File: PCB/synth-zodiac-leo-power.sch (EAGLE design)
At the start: 29 parts, among them J1 2.5 ID x 5.5 OD, J2 HDR-02P

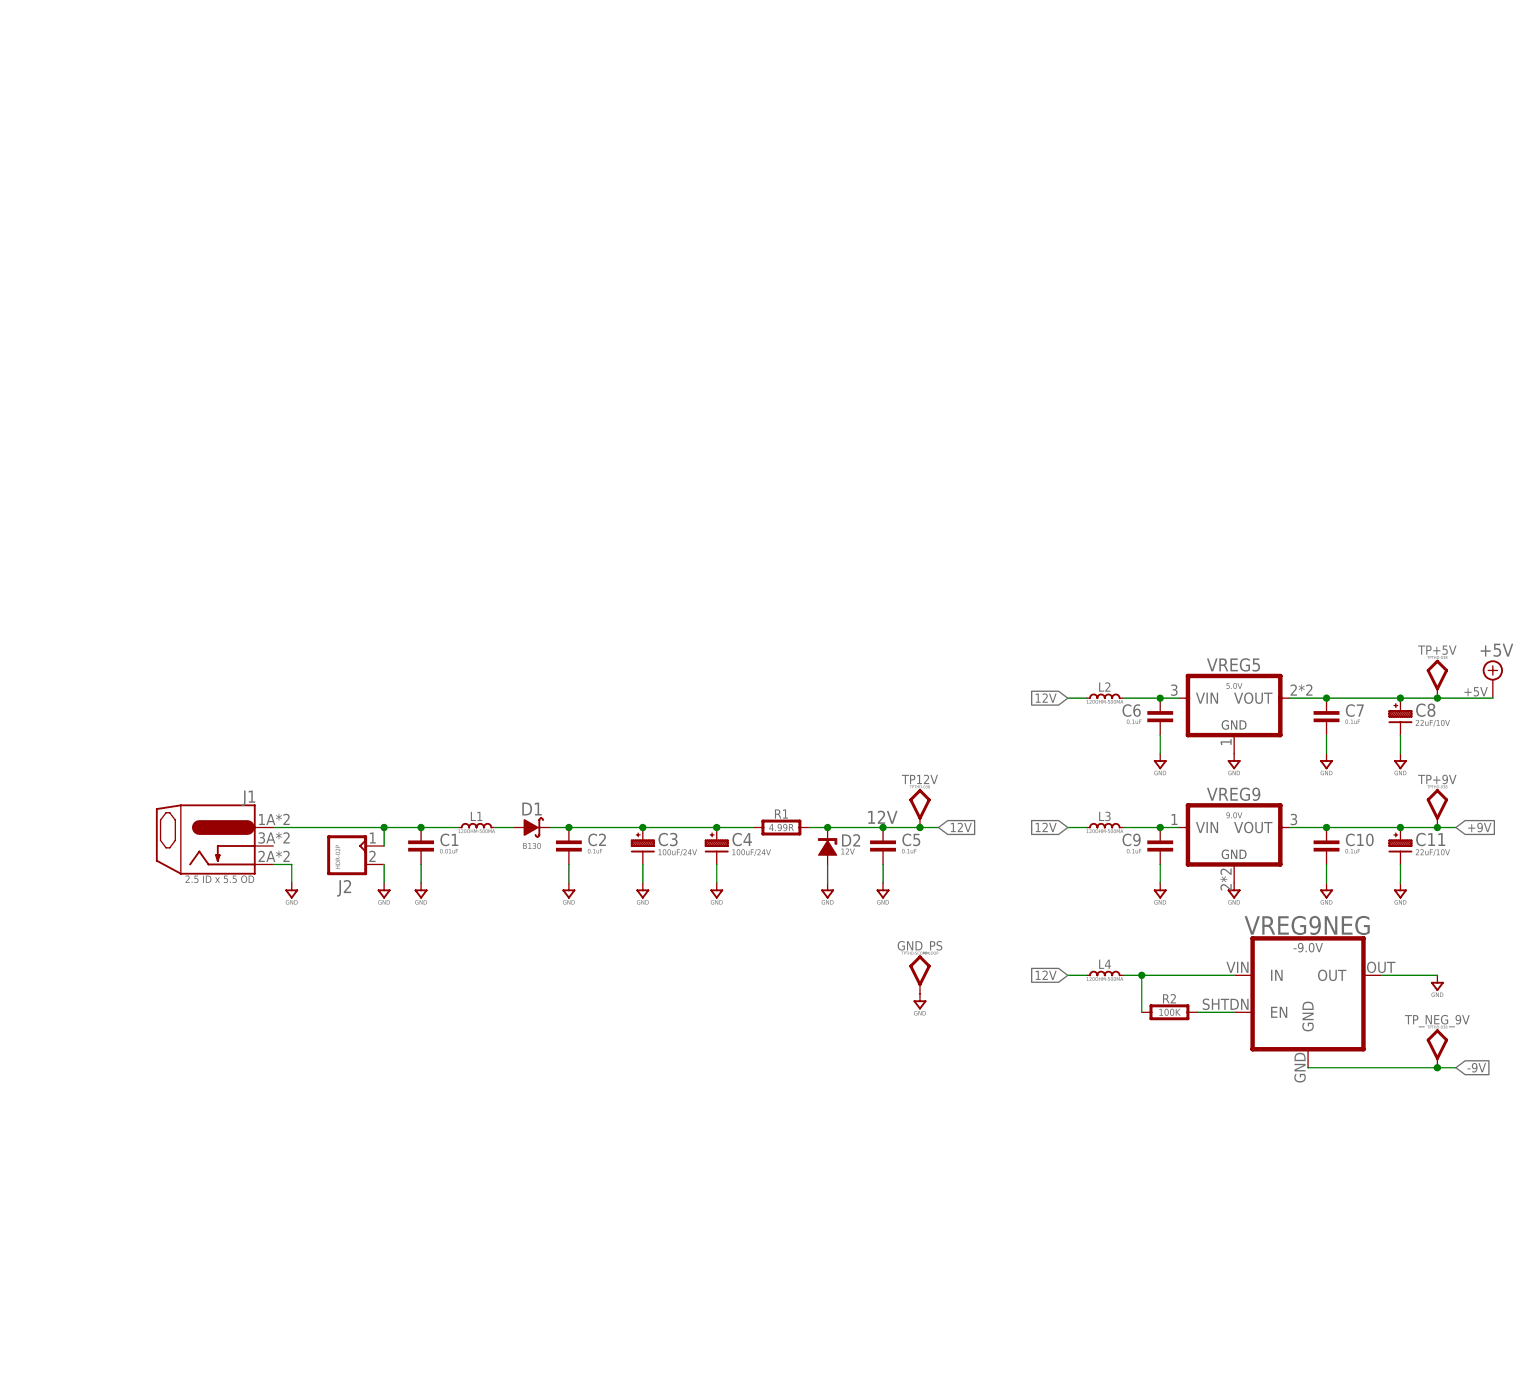
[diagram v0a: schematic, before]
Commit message: Snapshot of designs so far.
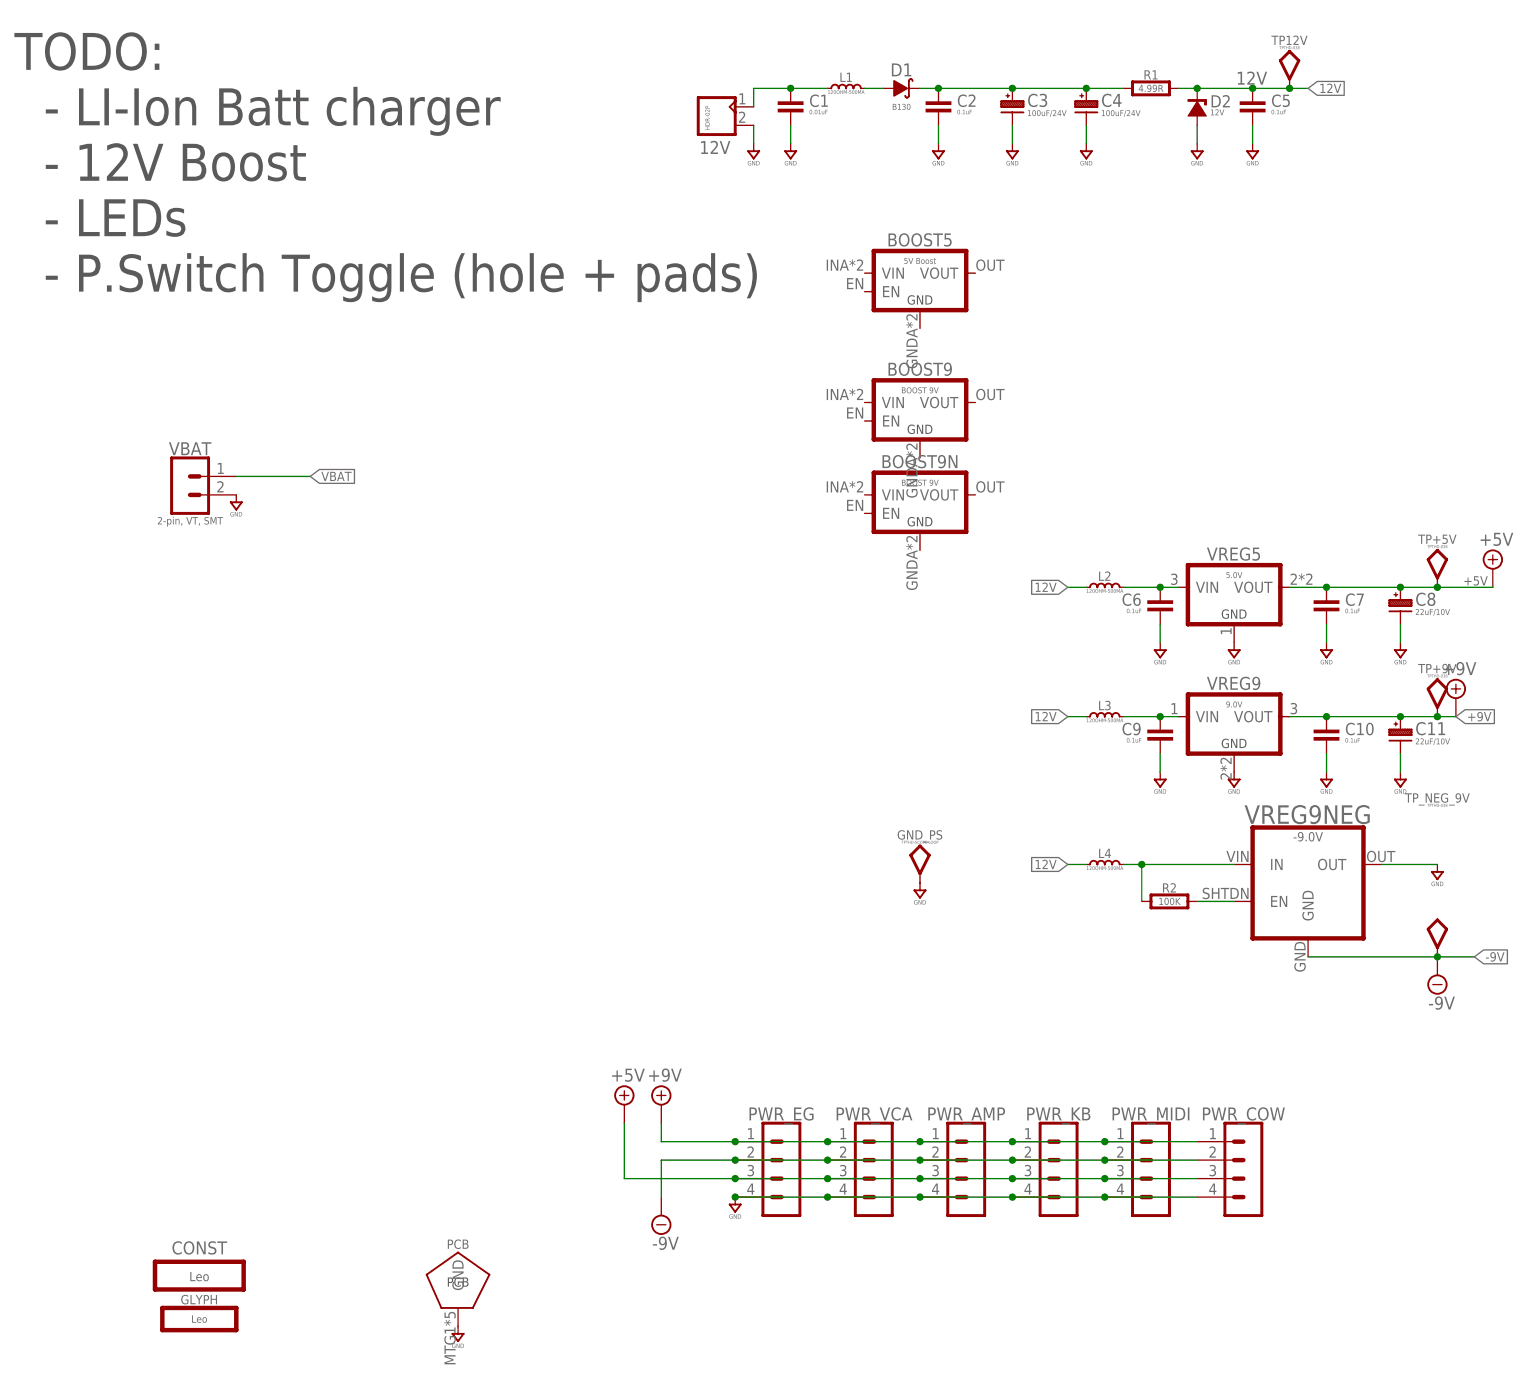
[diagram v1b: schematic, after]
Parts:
- removed J1: 2.5 ID x 5.5 OD, con-jack:DC-JACK-2.5MM-REGULAR
- removed J2: HDR-02P, con-headers:CON_02X1-2.54MM-THD-VT
- added 12V: HDR-02P, con-headers:CON_02X1-2.54MM-THD-VT
- added BOOST5: 5V Boost, regulators:BOOST-EN-POLOLU-5V
- added BOOST9, BOOST9N: BOOST 9V, regulators:BOOST-EN-POLOLU-9V
- added CONST: Leo, circuit-monkey-zodiac:CONSTELLATION-LEO
- added GLYPH: Leo, circuit-monkey-zodiac:GLYPH-LEO
- added PCB: PCB FAB, circuit-monkey-zodiac:PENTAGON-40R
- added PWR_AMP, PWR_COW, PWR_EG, PWR_KB, PWR_MIDI, PWR_VCA: (no value), con-jst:04P-VT-SMT
- added VBAT: 2-pin, VT, SMT, con-jst:02PVT-SMT
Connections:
- new net VBAT: VBAT.1
- net +5V: now also PWR_AMP.3, PWR_COW.3, PWR_EG.3, PWR_KB.3, PWR_MIDI.3, PWR_VCA.3
- net +9V: now also PWR_AMP.1, PWR_COW.1, PWR_EG.1, PWR_KB.1, PWR_MIDI.1, PWR_VCA.1
- net -9V: now also PWR_AMP.2, PWR_COW.2, PWR_EG.2, PWR_KB.2, PWR_MIDI.2, PWR_VCA.2
- net GND: now also 12V.2, PCB.GND@1, PWR_AMP.4, PWR_COW.4, PWR_EG.4, PWR_KB.4, PWR_MIDI.4, PWR_VCA.4, VBAT.2; no longer J1.GND, J2.2
- net N$1: now also 12V.1; no longer J1.VIN, J2.1
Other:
- note added: "TODO: - LI-Ion Batt charger - 12V Boost - LEDs - P.Switch Toggle (hole + pads)"
- moved on the sheet: C1, C10, C11, C2, C3, C4, C5, C6, C7, C8, C9, D1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
